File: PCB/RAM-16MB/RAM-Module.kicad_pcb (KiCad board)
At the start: 4 copper layers, 41.5 x 41.6 mm, 22 parts, among them J15 RAM Module, U1 51W17800TT6, U2 51W17800TT6, U3 51W17800TT6, U4 51W17800TT6, U5 51W17800TT6, U6 51W17800TT6, U7 51W17800TT6, U8 51W17800TT6

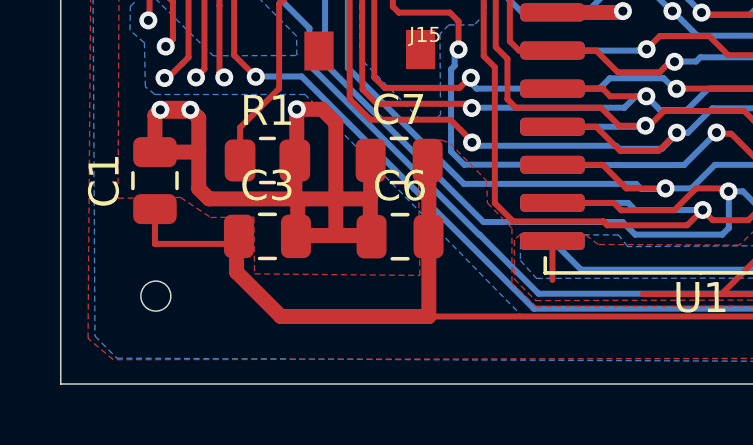
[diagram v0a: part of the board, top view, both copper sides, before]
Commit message: Add files via upload
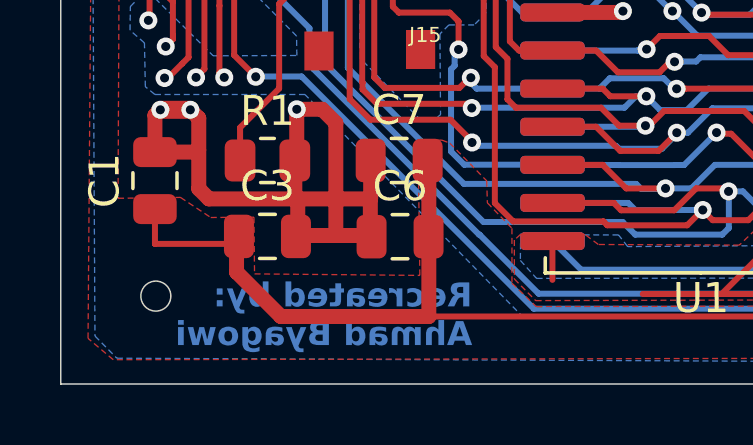
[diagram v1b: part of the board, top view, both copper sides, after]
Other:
- board text added: "Recreated by: Ahmad Byagowi"
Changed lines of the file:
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@@
 		(layer "Edge.Cuts")
+	)
+	(gr_text "Recreated by:\nAhmad Byagowi"
+		(at 122.78 118.82 0)
+		(layer "B.Cu" knockout)
+		(effects
+			(font
+				(size 0.8 0.8)
+				(thickness 0.175)
+				(bold yes)
+			)
+			(justify left bottom mirror)
+		)
 	)
 	(segment
